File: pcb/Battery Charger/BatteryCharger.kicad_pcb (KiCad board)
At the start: 2 copper layers, 20 x 37.4 mm, 24 parts, among them Q1 FS8205A, U1 DW01A, U3 MCP73831

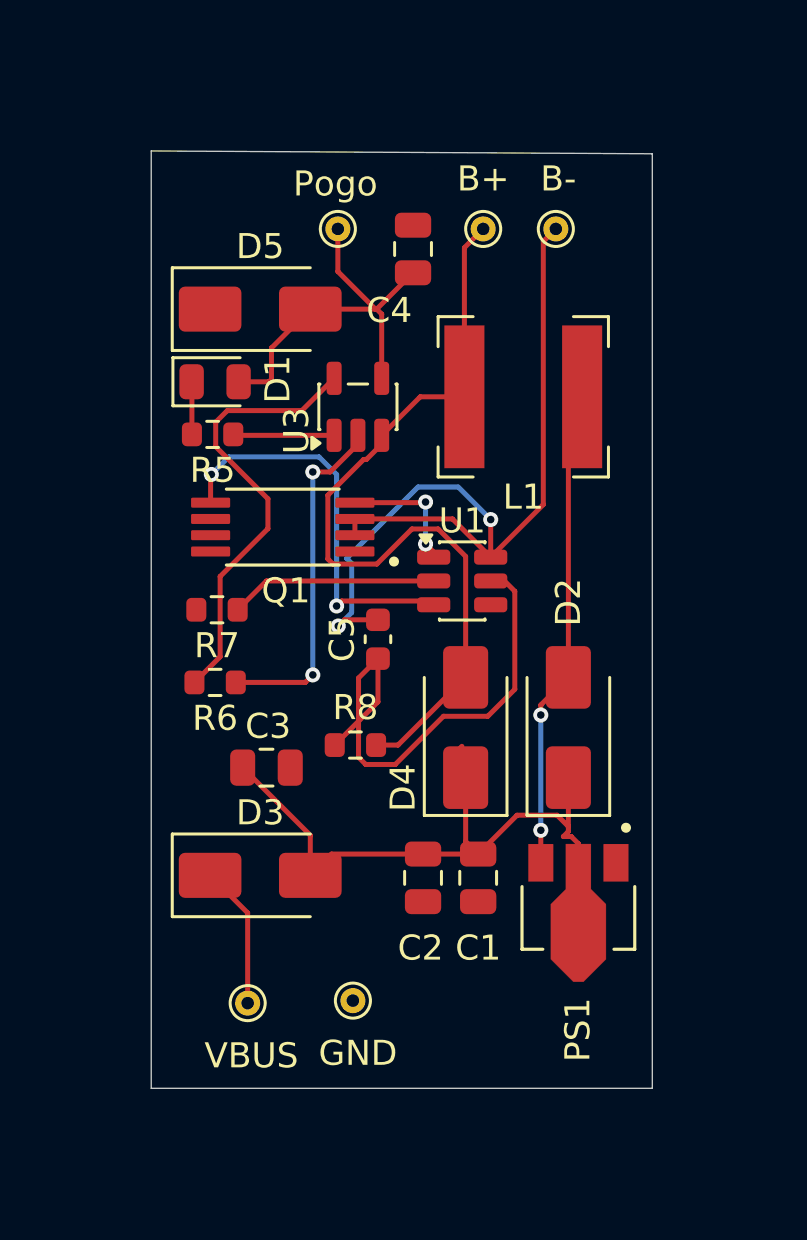
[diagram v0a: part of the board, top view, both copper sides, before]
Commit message: charger has been finished final draft
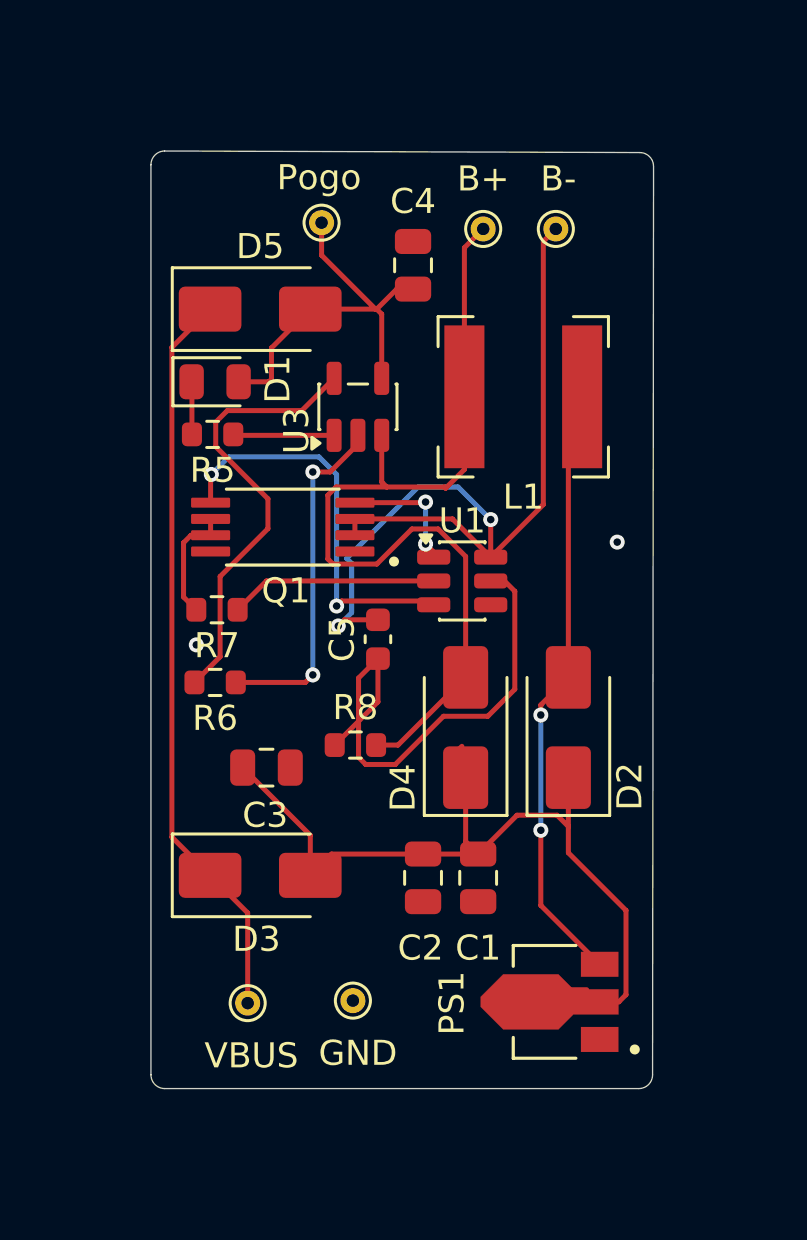
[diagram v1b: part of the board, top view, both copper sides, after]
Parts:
- moved PS1 3.73 mm to (198.7, 87.2), turned to 180 degrees
- moved Pogo 0.70 mm to (189.6, 56.0)
- moved C4 0.65 mm to (193.2, 57.8)
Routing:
- net Net-(D3-K): track 5.72 -> 29.6 mm
- net Net-(D2-K): track 25.2 -> 32.8 mm
- net Net-(D2-A): track 19.3 -> 24.3 mm
- net GND: track 14.1 -> 18.9 mm, vias 2 -> 4
- net Net-(D4-A): track 33.2 -> 36.8 mm
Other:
- board size 20 x 37.4 mm -> 20.1 x 37.4 mm
